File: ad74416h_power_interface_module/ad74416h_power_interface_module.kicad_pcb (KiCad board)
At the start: 4 copper layers, 55.9 x 40.6 mm, 123 parts, among them J1 FW-33-03-G-D-085-155, T1 ZA9644-AED, U1 MAX17227JATA+, U2 MAX17614ATP+, U3 MAX17570FATA+, U4 ADP1031ACPZ-3-R7, U5 ADUM340E0BRQZ, U6 ADUM340E0BRQZ, U7 ADUM1252AUA+

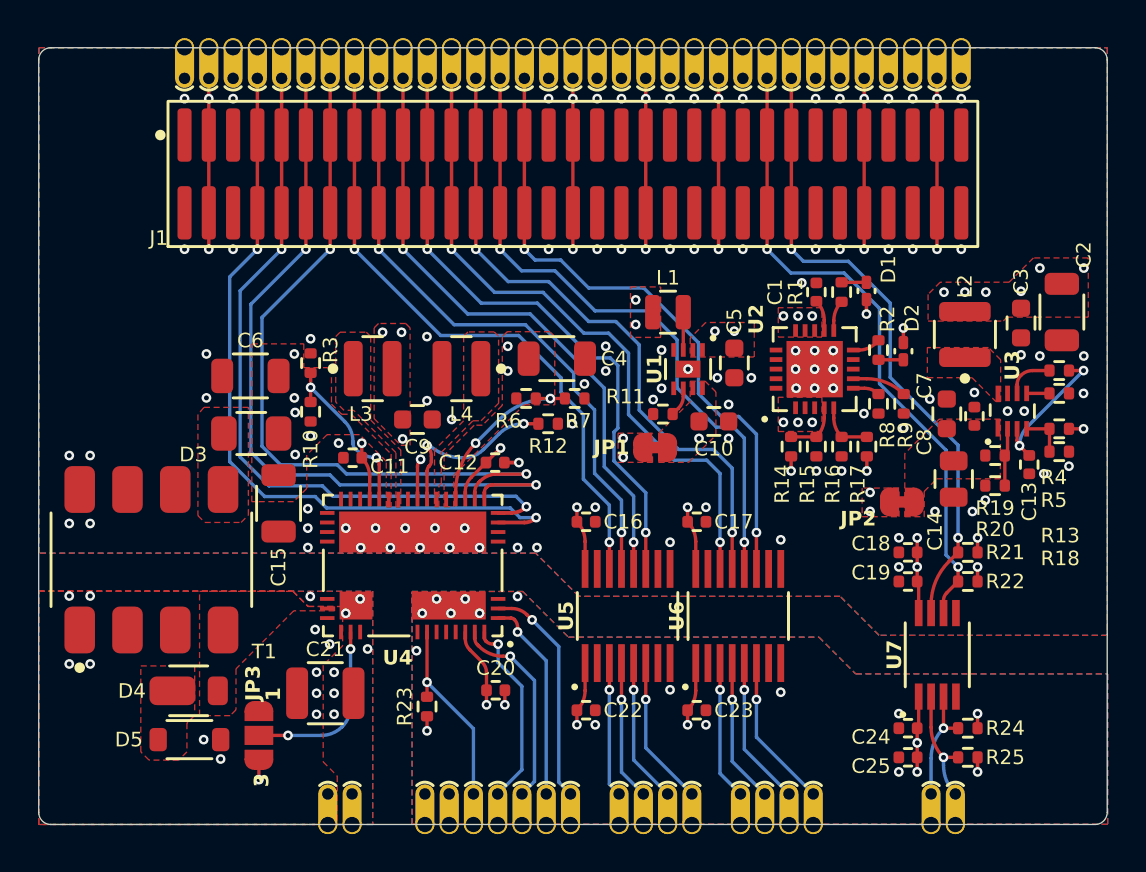
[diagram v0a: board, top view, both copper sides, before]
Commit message: backup
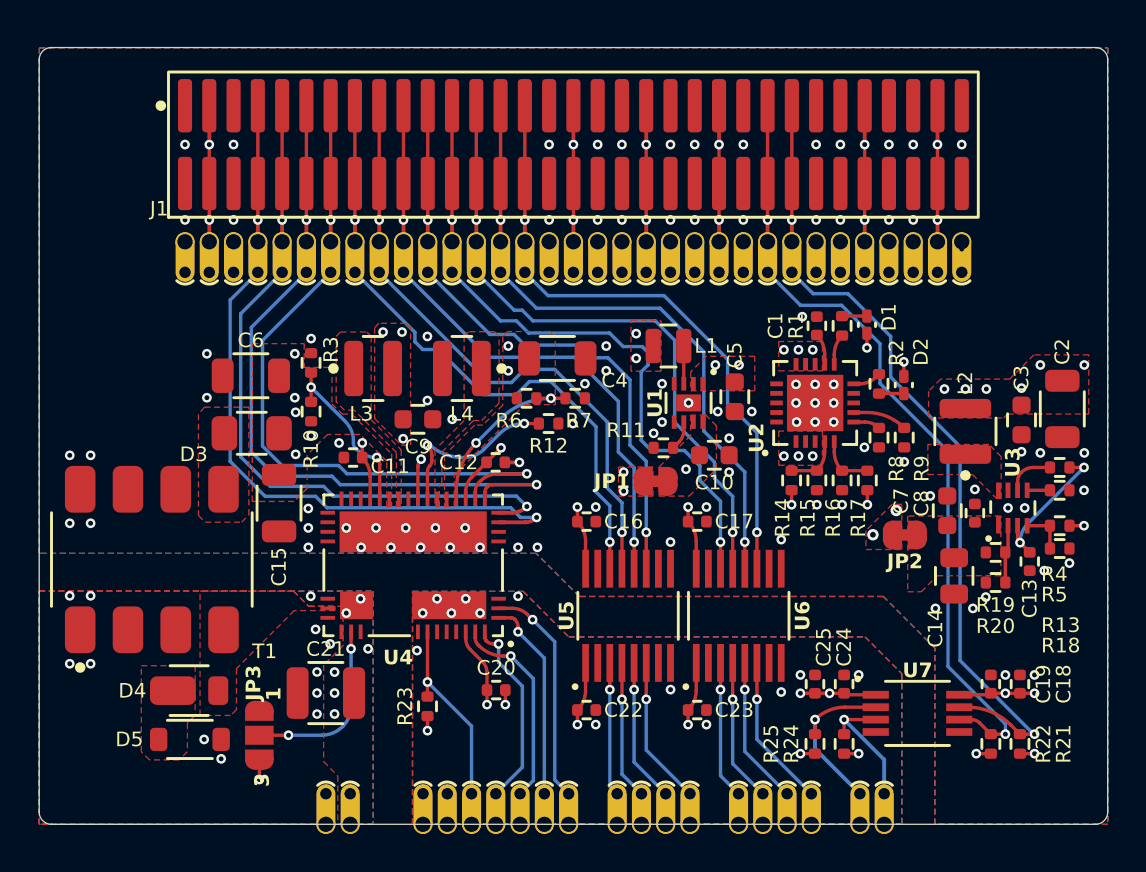
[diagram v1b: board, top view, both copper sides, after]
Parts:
- moved R21 10.4 mm to (168.1, 115.2), turned to 90 degrees
- moved TP1 10.1 mm to (124.4, 88.9)
- moved TP10 10.1 mm to (135.9, 88.9)
- moved TP11 10.1 mm to (137.1, 88.9)
- moved TP12 10.1 mm to (138.4, 88.9)
- moved TP13 10.1 mm to (139.7, 88.9)
- moved TP14 10.1 mm to (141.0, 88.9)
- moved TP15 10.1 mm to (142.2, 88.9)
- moved TP16 10.1 mm to (143.5, 88.9)
- moved TP17 10.1 mm to (144.8, 88.9)
- moved TP18 10.1 mm to (146.0, 88.9)
- moved TP19 10.1 mm to (147.3, 88.9)
- moved TP2 10.1 mm to (125.7, 88.9)
- moved TP20 10.1 mm to (152.4, 88.9)
- moved TP21 10.1 mm to (149.8, 88.9)
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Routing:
- net /SDA: track 33.4 -> 42.0 mm
- net /SCL: track 34.0 -> 40.4 mm
- net /2B1: track 34.4 -> 30.3 mm
- net /SDI: track 39.6 -> 36.6 mm
- net /~{SYNC}: track 39.9 -> 36.9 mm
- net /SCLK: track 38.7 -> 35.7 mm
- net /SDO: track 38.3 -> 35.3 mm
- net /SDA_ISO: track 6.17 -> 8.96 mm
- net /1B1: track 33.7 -> 31.2 mm
- net /1B2: track 34.1 -> 31.7 mm
- net /2B2: track 32.6 -> 30.3 mm
- net /2B3: track 33.1 -> 30.9 mm
- net /1B3: track 34.4 -> 32.2 mm
- net /2B4: track 33.6 -> 31.7 mm
- net /3V3: track 31.2 -> 29.3 mm
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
